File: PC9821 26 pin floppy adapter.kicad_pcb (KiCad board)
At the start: 2 copper layers, 31 x 54.4 mm, 3 parts

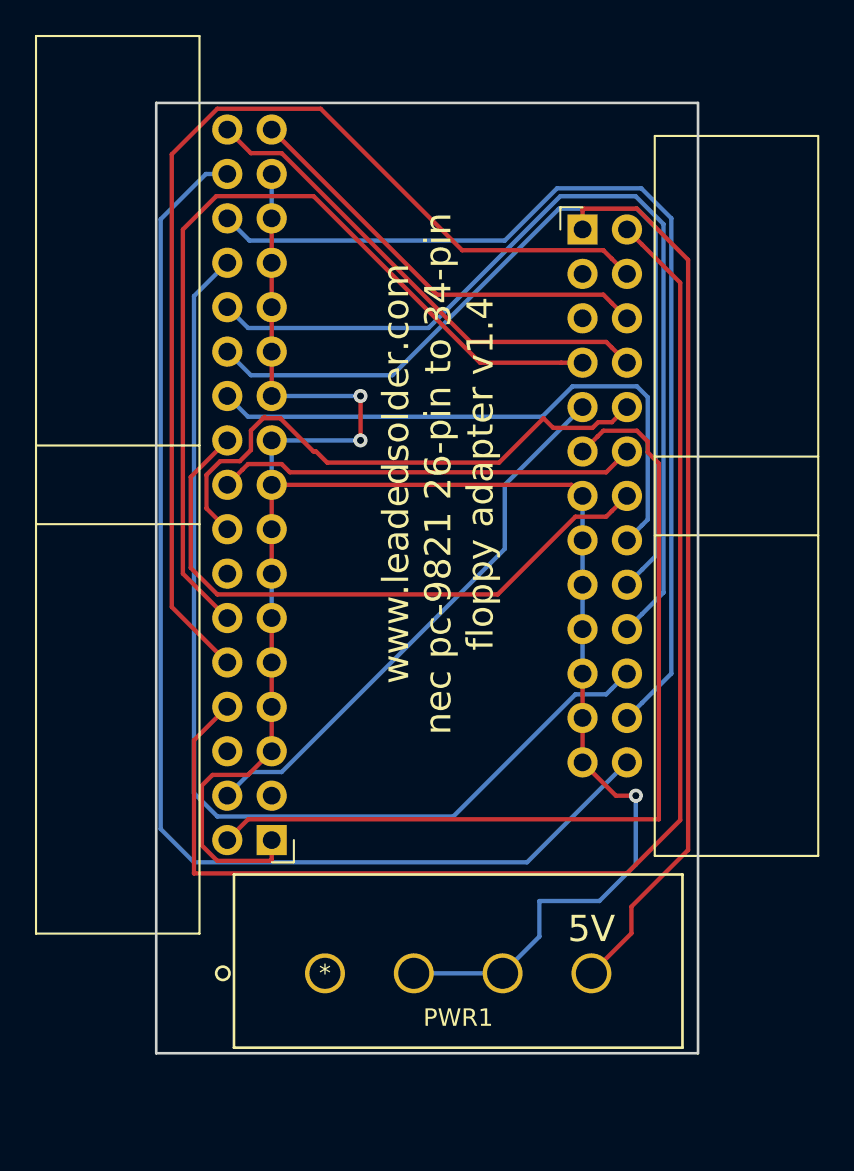
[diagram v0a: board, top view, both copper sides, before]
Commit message: v1.5 revision
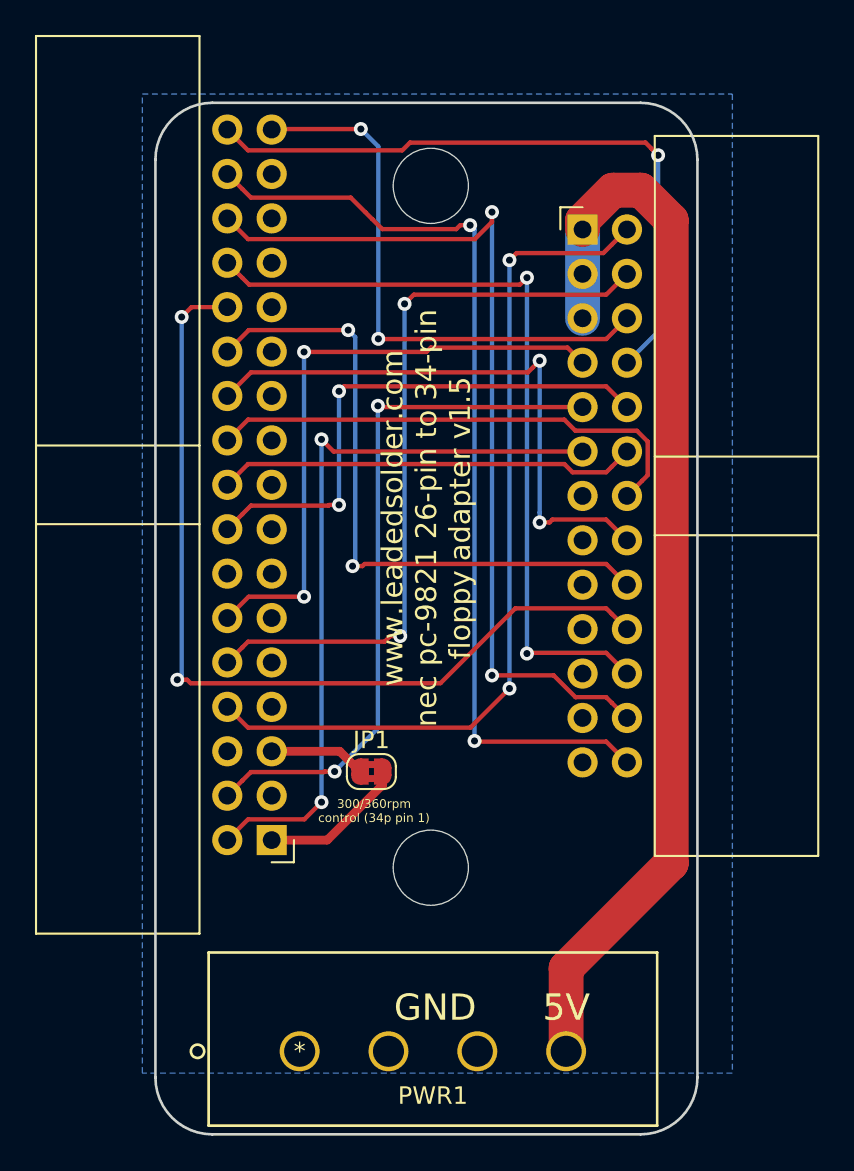
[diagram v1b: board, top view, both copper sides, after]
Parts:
- added G***: LOGO, Logos:pi-rat-small, B.Cu at (158.8, 104.5)
- added JP1: 300/360 control, Jumper:SolderJumper-2_P1.3mm_Bridged2Bar_RoundedPad1.0x1.5mm, F.Cu at (158.1, 118.0)
- added REF**: MountingHole_4.3mm_M4, MountingHole:MountingHole_4.3mm_M4, F.Cu at (161.5, 84.5)
- added REF**: MountingHole_4.3mm_M4, MountingHole:MountingHole_4.3mm_M4, F.Cu at (161.5, 123.5)
- moved PWR1 4.69 mm to (154.0, 134.0)
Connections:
- GOTEK1 pad 11: /360_300_DRV_0 -> /GND
- GOTEK1 pad 13: /360_300_DRV_0 -> /GND
- GOTEK1 pad 15: /360_300_DRV_0 -> /GND
- GOTEK1 pad 17: /360_300_DRV_0 -> /GND
- GOTEK1 pad 19: /360_300_DRV_0 -> /GND
- GOTEK1 pad 21: /360_300_DRV_0 -> /GND
- GOTEK1 pad 23: /360_300_DRV_0 -> /GND
- GOTEK1 pad 25: /360_300_DRV_0 -> /GND
- GOTEK1 pad 27: /360_300_DRV_0 -> /GND
- GOTEK1 pad 29: /360_300_DRV_0 -> /GND
- GOTEK1 pad 31: /360_300_DRV_0 -> /GND
- GOTEK1 pad 5: /360_300_DRV_0 -> /GND
- GOTEK1 pad 7: /360_300_DRV_0 -> /GND
- GOTEK1 pad 9: /360_300_DRV_0 -> /GND
- PC98-F1 pad 13: /360_300_DRV_0 -> /GND
- PC98-F1 pad 15: /360_300_DRV_0 -> /GND
- PC98-F1 pad 17: /360_300_DRV_0 -> /GND
- PC98-F1 pad 19: /360_300_DRV_0 -> /GND
- PC98-F1 pad 21: /360_300_DRV_0 -> /GND
- PC98-F1 pad 23: /360_300_DRV_0 -> /GND
- PC98-F1 pad 25: /360_300_DRV_0 -> /GND
- PC98-F1 pad 3: /+5V_2 -> /+5V_1
- PC98-F1 pad 5: /+5V_3 -> /+5V_1
- PWR1 pad 2: /360_300_DRV_0 -> /GND
- PWR1 pad 3: /360_300_DRV_0 -> /GND
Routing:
- net /360_300_DRV_0: track 114.4 -> 8.41 mm, vias 3 -> 0
- net /INDEX_OUT: track 74.4 -> 49.5 mm, vias 0 -> 2
- net /DRV_SELECT_0: track 61.4 -> 43.0 mm, vias 0 -> 2
- net /DRV_SELECT_1: track 50.9 -> 35.3 mm, vias 0 -> 2
- net /SIDE: track 69.6 -> 54.1 mm, vias 0 -> 2
- net /WRITE_PROTECT: track 59.8 -> 45.6 mm, vias 0 -> 2
- net /WRITE_ENABLE: track 50.6 -> 37.4 mm, vias 0 -> 2
- net /+5V_1: track 51.5 -> 62.1 mm
- net /READY_OUT: track 28.4 -> 38.6 mm, vias 0 -> 1
- net /DENSITY: track 51.5 -> 42.3 mm, vias 0 -> 2
- net /HEAD_LOAD: track 31.7 -> 40.4 mm, vias 0 -> 2
- net /DISK_CHANGE: track 24.8 -> 32.6 mm, vias 0 -> 2
- net /STEP_PULSE: track 36.1 -> 28.7 mm
- net /READ_DATA: track 57.5 -> 51.8 mm, vias 0 -> 2
- net /GND: track 0.00 -> 5.53 mm
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- added copper zone on B.Cu, net /GND
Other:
- board size 31 x 54.4 mm -> 31 x 59 mm
- board text added: "300/360rpm control (34p pin 1)"
- board text added: "GND"
- board text added: "www.leadedsolder.com nec pc-9821 26-pin to 34-pin floppy adapter v1.5"
- board text removed: "www.leadedsolder.com nec pc-9821 26-pin to 34-pin floppy adapter v1.4"
